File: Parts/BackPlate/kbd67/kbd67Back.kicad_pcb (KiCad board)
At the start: 2 copper layers, 172.9 x 20 mm, 3 parts

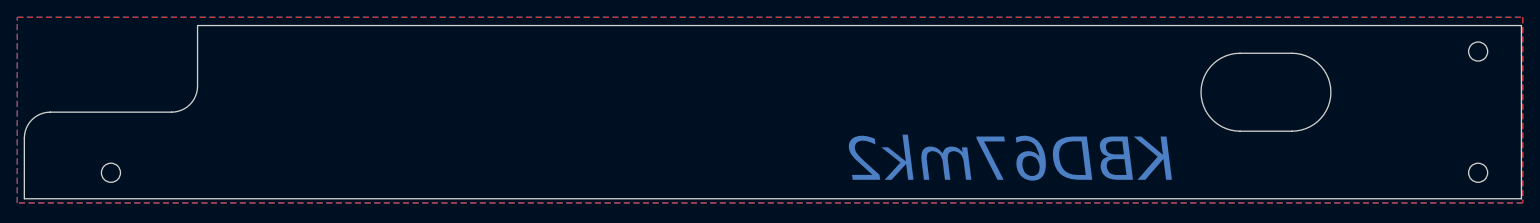
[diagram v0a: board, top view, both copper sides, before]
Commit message: 寸法更新とか
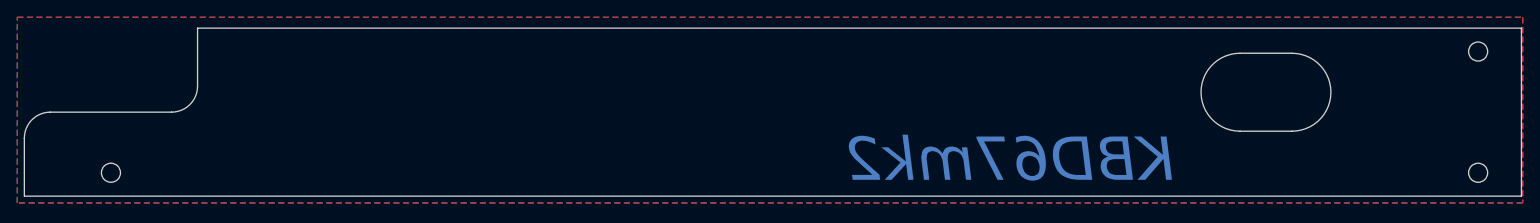
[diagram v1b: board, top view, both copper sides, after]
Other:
- board size 172.9 x 20 mm -> 172.9 x 19.4 mm
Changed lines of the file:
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@@
   (gr_line (start 279.3 23.2) (end 285.3 23.2) (layer Edge.Cuts) (width 0.1))
   (gr_line (start 285.3 32.2) (end 279.3 32.2) (layer Edge.Cuts) (width 0.1))
-  (gr_line (start 311.8 20) (end 158.925 20) (layer Edge.Cuts) (width 0.1))
-  (gr_line (start 311.8 40) (end 138.925 40) (layer Edge.Cuts) (width 0.1))
+  (gr_line (start 311.8 20.3) (end 158.925 20.3) (layer Edge.Cuts) (width 0.1))
+  (gr_line (start 311.8 39.7) (end 138.925 39.7) (layer Edge.Cuts) (width 0.1))
   (gr_arc (start 141.925 33) (end 141.925 30) (angle -90) (layer Edge.Cuts) (width 0.1))
   (gr_arc (start 155.925 27) (end 155.925 30) (angle -90) (layer Edge.Cuts) (width 0.1))
-  (gr_line (start 138.925 33) (end 138.925 40) (layer Edge.Cuts) (width 0.1))
+  (gr_line (start 138.925 33) (end 138.925 39.7) (layer Edge.Cuts) (width 0.1))
   (gr_line (start 155.925 30) (end 141.925 30) (layer Edge.Cuts) (width 0.1))
-  (gr_line (start 158.925 20) (end 158.925 27) (layer Edge.Cuts) (width 0.1))
-  (gr_line (start 311.8 40) (end 311.8 20) (layer Edge.Cuts) (width 0.1))
+  (gr_line (start 158.925 20.3) (end 158.925 27) (layer Edge.Cuts) (width 0.1))
+  (gr_line (start 311.8 39.7) (end 311.8 20.3) (layer Edge.Cuts) (width 0.1))
   (zone (net 0) (net_name "") (layer F.Cu) (hatch edge 0.508)
     (connect_pads (clearance 0.508))
